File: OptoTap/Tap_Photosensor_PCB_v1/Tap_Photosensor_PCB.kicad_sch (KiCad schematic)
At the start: 7 parts, among them J1 Conn_01x01_Male, J2 Conn_01x01_Male, J3 Conn_01x01_Male, U1 OPB961N51

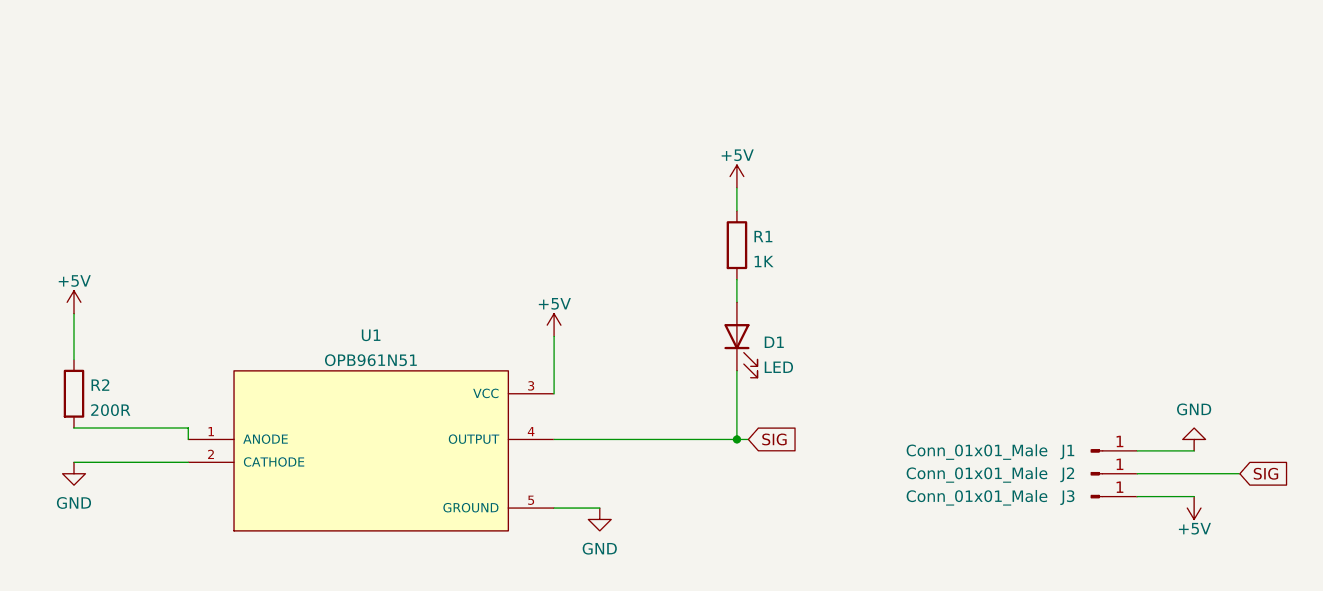
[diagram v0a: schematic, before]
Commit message: updated OptoTap boards
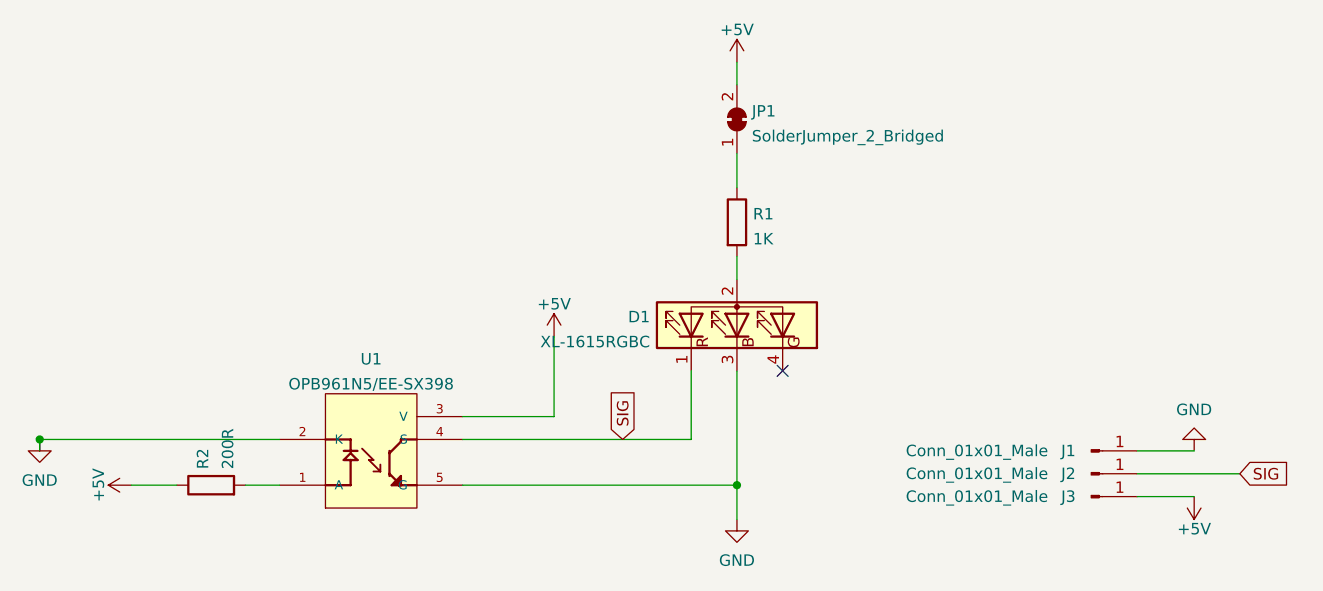
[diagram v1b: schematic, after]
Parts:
- removed D1: LED, LED_SMD:LED_0805_2012Metric, symbol Device:LED
- added D1: XL-1615RGBC, LED_SMD:LED_0606_1432, symbol LED:XL-1615RBGC
- added JP1: SolderJumper_2_Bridged, Jumper:SolderJumper-2_P1.3mm_Bridged_RoundedPad1.0x1.5mm, symbol Jumper:SolderJumper_2_Bridged
- R1: LCSC (none) -> C17513
- R2: LCSC (none) -> C17540
- U1: value OPB961N51 -> OPB961N5/EE-SX398; footprint OPTO_OPB961N51 -> footprints:OPTO_EE-SX398_OPB666N; symbol OPB961N51:OPB961N51 -> EE-SX398:EE-SX398_OPBxxx; MANUFACTURER TT Electronics -> Omron; MAXIMUM_PACKAGE_HEIGHT 10.8mm -> 10.2 mm; PARTREV D -> NA; STANDARD IPC-7351B -> Manufacturer Recommendations
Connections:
- net +5V: now also JP1.2 (B); no longer R1.1
- net GND: now also D1.3 (B)
- net SIG: now also D1.1 (R)
- net at R1.2: now also D1.2 (A)
- new net: JP1.1 (A), R1.1
- no-connect marks 0 -> 1
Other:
- moved on the sheet: R1, R2
